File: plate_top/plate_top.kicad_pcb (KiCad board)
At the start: 2 copper layers, 173.5 x 138.9 mm, 46 parts, among them SW1 SW_Push, SW10 SW_Push, SW11 SW_Push, SW12 SW_Push, SW13 SW_Push, SW14 SW_Push, SW15 SW_Push, SW16 SW_Push, SW17 SW_Push, SW18 SW_Push, SW19 SW_Push, SW2 SW_Push, SW20 SW_Push, SW21 SW_Push, SW22 SW_Push, SW23 SW_Push, SW24 SW_Push, SW25 SW_Push, SW26 SW_Push, SW27 SW_Push, SW28 SW_Push, SW29 SW_Push, SW3 SW_Push, SW30 SW_Push, SW31 SW_Push, SW32 SW_Push, SW4 SW_Push, SW5 SW_Push, SW6 SW_Push, SW7 SW_Push, SW8 SW_Push, SW9 SW_Push

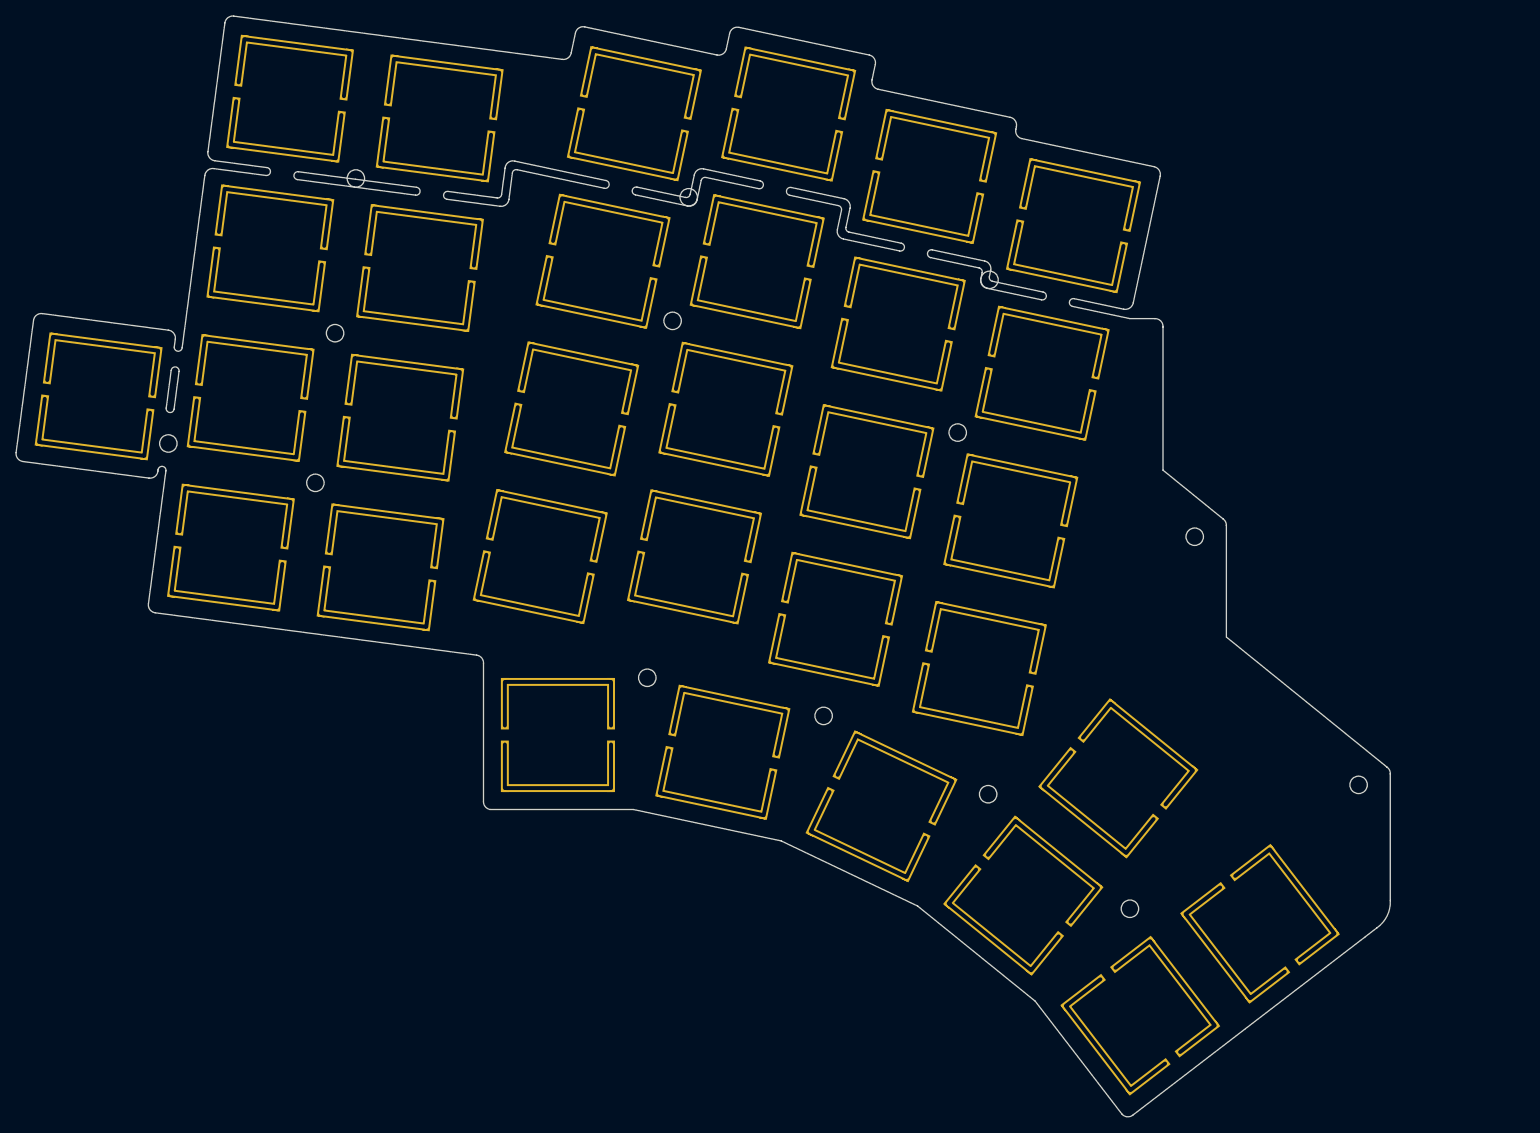
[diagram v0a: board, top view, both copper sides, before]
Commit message: Holes and top plate
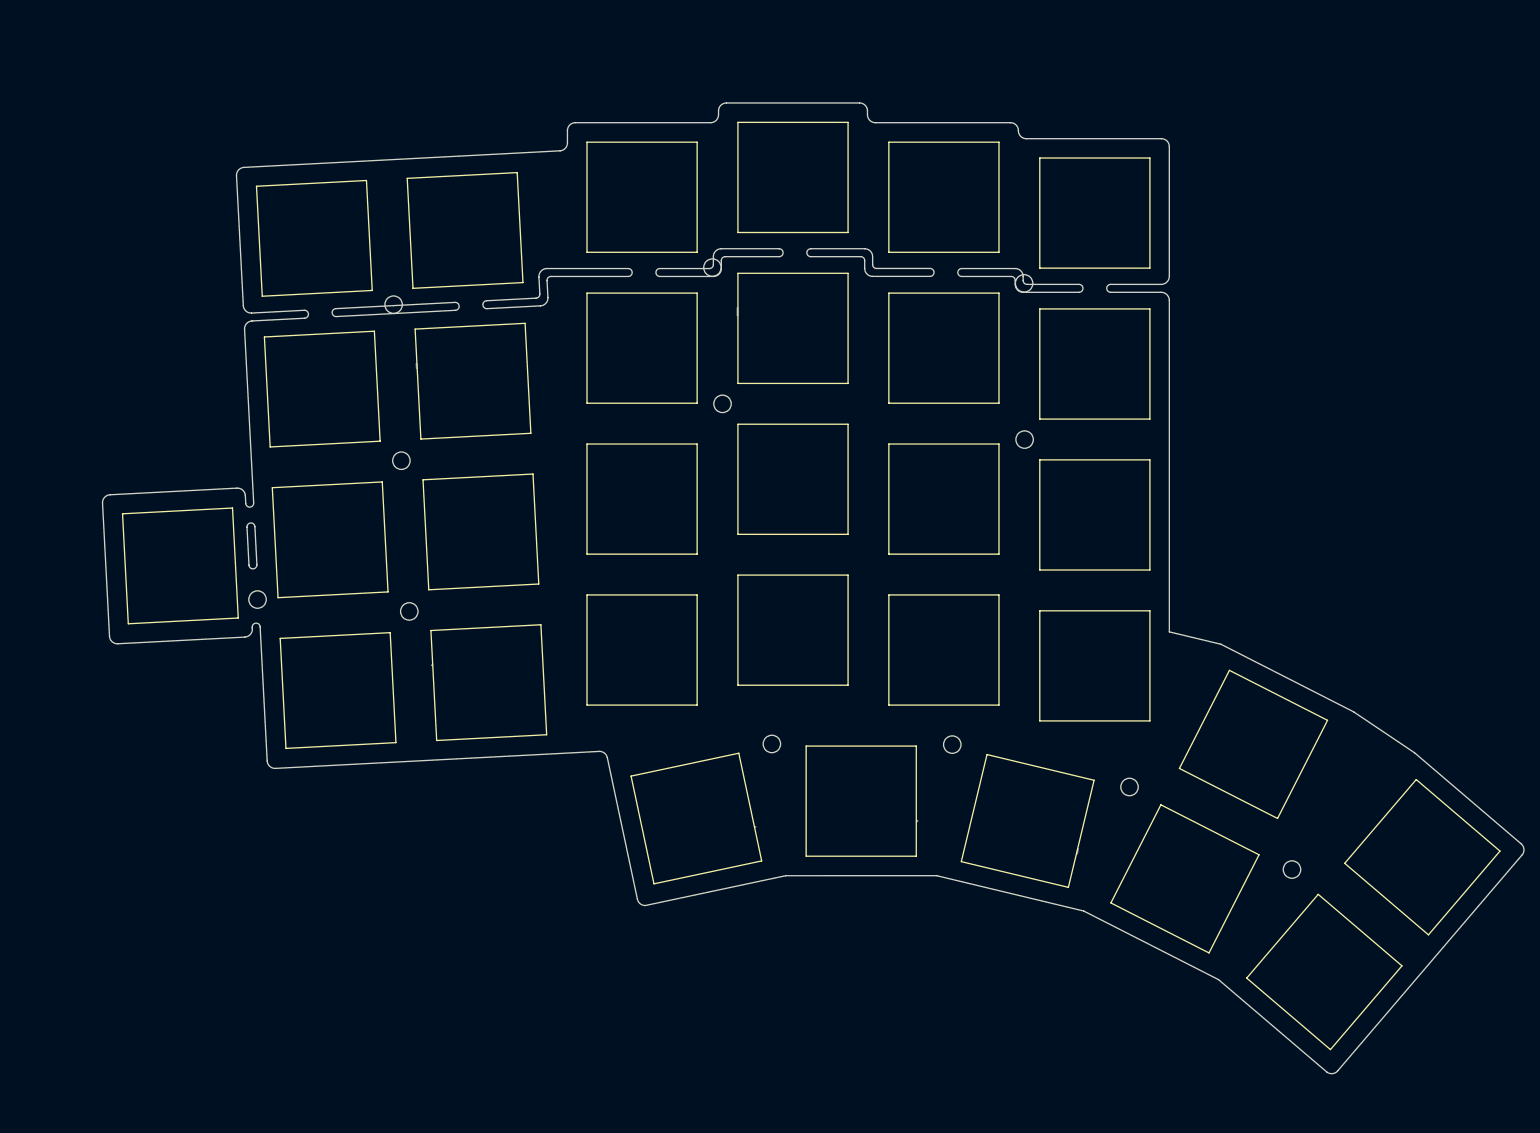
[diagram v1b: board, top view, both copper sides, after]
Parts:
- removed H16: MountingHole, used_footprints:M2_HOLE_PCB
- removed HM1: CaseHole, used_footprints:M2_HOLE_PCB
- SW1, SW10, SW11, SW12, SW13, SW14, SW15, SW16, SW17, SW18, SW19, SW2, SW20, SW21, SW22, SW23, SW24, SW25, SW26, SW27, SW28, SW29, SW3, SW30, SW31, SW32, SW4, SW5, SW6, SW7, SW8, SW9: footprint used_footprints:metallized_breakout_cutout -> used_footprints:CherryMX_Hole_for_layout_tester
- moved SW32 23.9 mm to (218.4, 140.8), turned to 319.5 degrees
- moved SW27 23.8 mm to (74.0, 89.6), turned to 183 degrees
- moved HM5 22.7 mm to (83.8, 93.8), turned to 3 degrees
- moved SW20 22.5 mm to (93.9, 105.3), turned to 183 degrees
- moved SW19 22.1 mm to (230.8, 126.3), turned to 139.5 degrees
- moved HM3 21.0 mm to (214.3, 127.9), turned to 4.5 degrees
- moved SW13 20.5 mm to (92.9, 86.3), turned to 183 degrees
- moved SW31 20.5 mm to (200.8, 129.1), turned to 333 degrees
- moved SW28 20.4 mm to (139.2, 121.5), turned to 12 degrees
- moved HM6 20.1 mm to (102.9, 95.3), turned to 3 degrees
- moved SW21 20.0 mm to (113.0, 104.3), turned to 183 degrees
- moved SW7 18.9 mm to (91.9, 67.3), turned to 183 degrees
- moved SW30 18.5 mm to (181.0, 121.8), turned to 346.5 degrees
- moved SW29 18.5 mm to (160.0, 119.3), turned to 0 degrees
- moved HM8 18.1 mm to (101.9, 76.3), turned to 3 degrees
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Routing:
- net (no net): track 0.00 -> 2.48 mm
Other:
- board size 173.5 x 138.9 mm -> 179.4 x 122.5 mm
